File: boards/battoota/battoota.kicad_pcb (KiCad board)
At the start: 2 copper layers, 122.6 x 88.9 mm, 38 parts

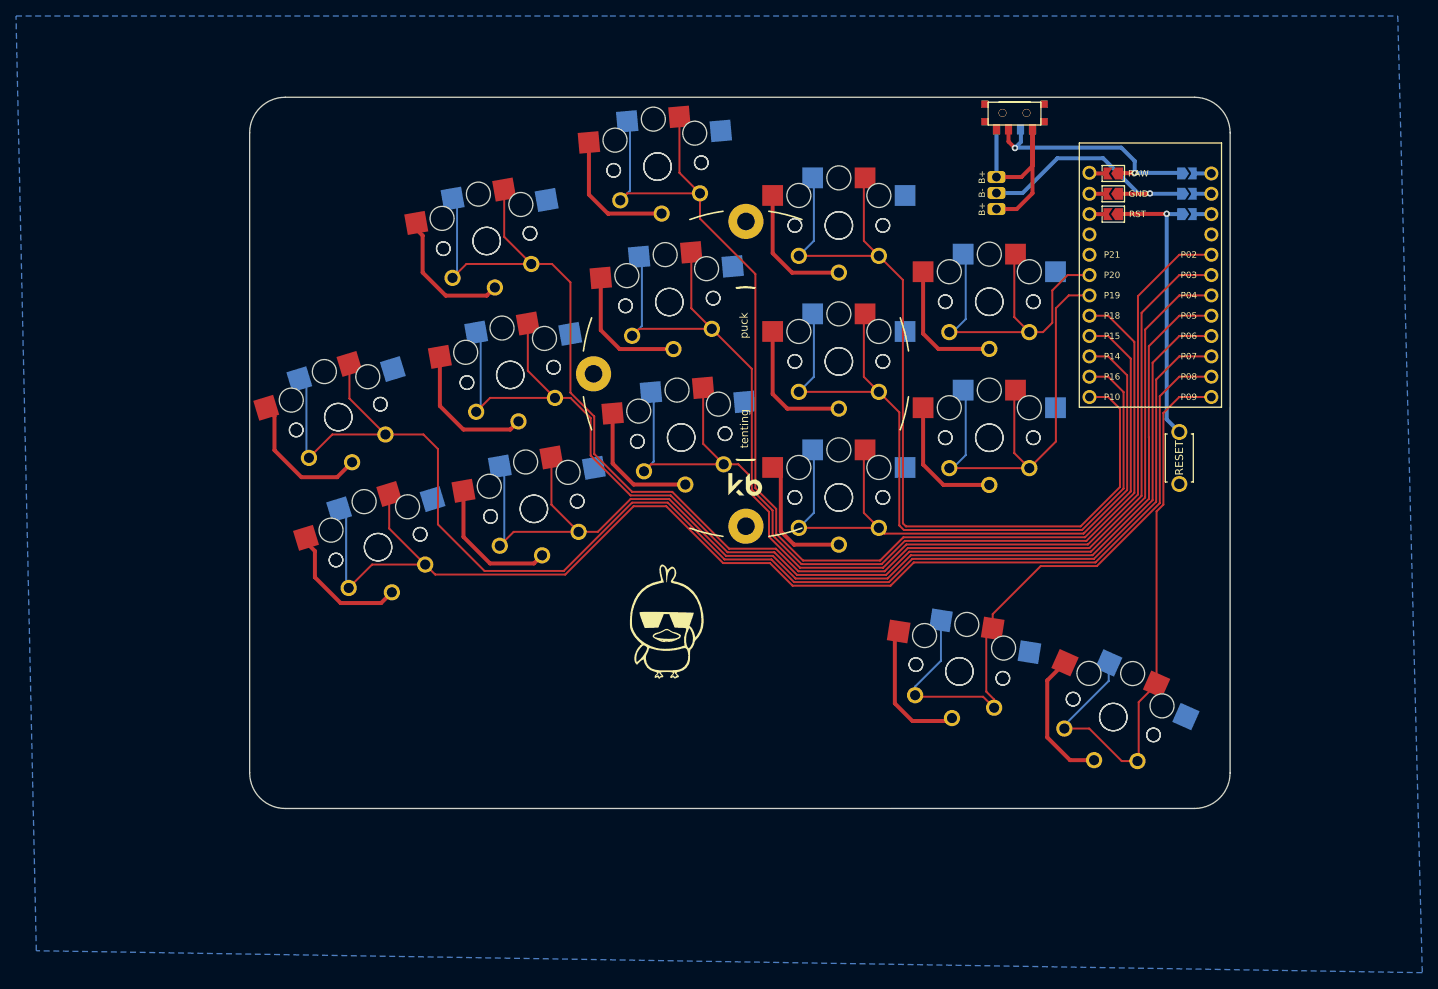
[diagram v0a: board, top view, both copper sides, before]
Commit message: battoota clean up
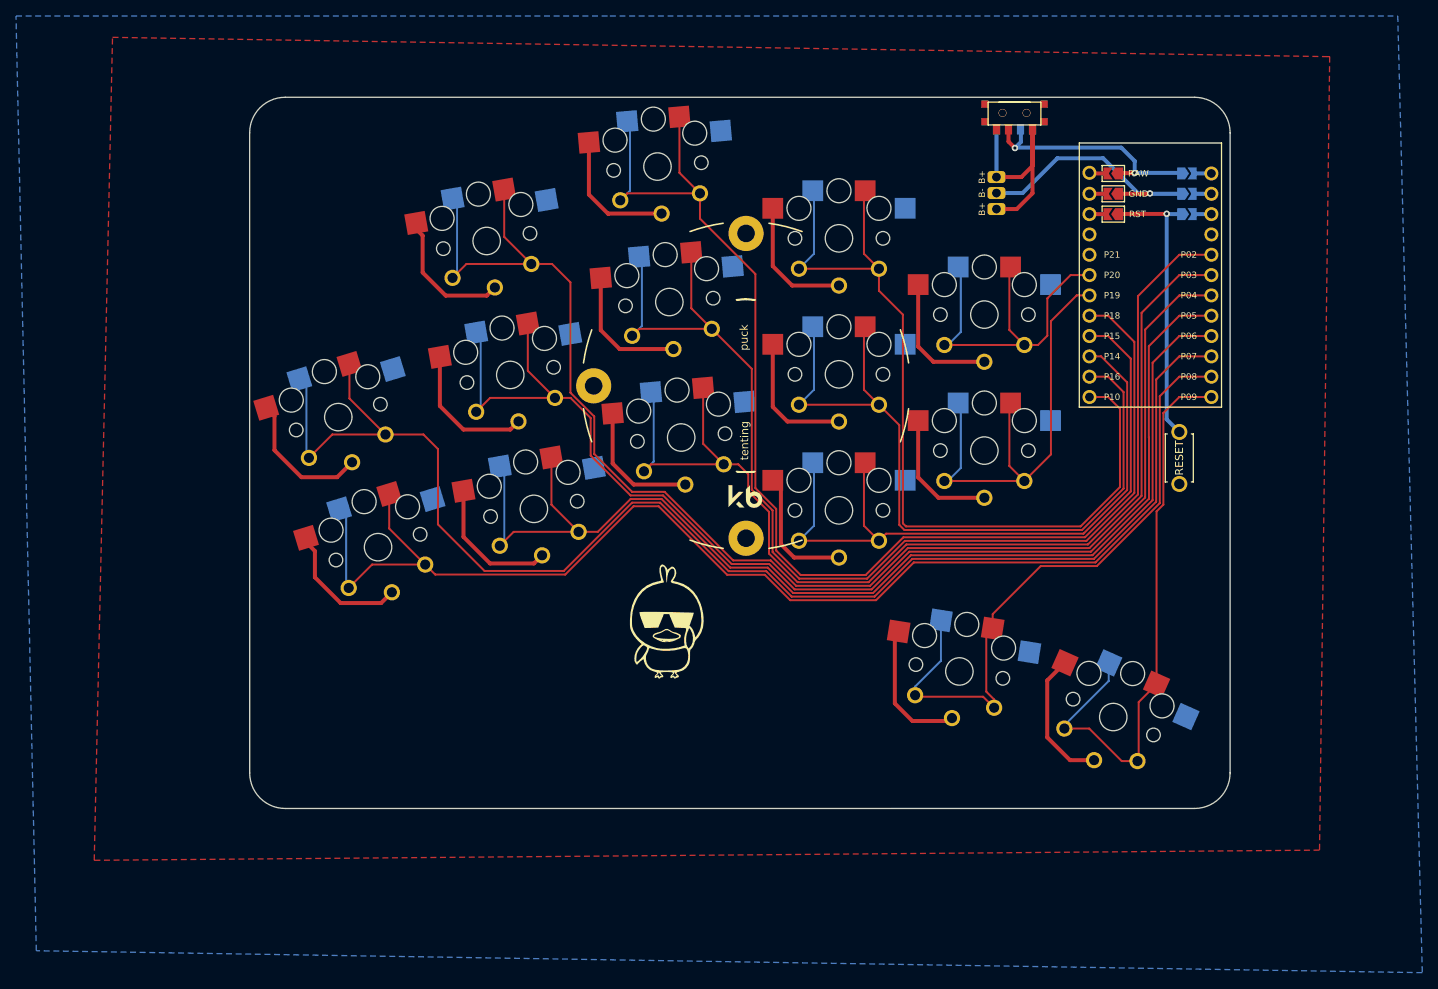
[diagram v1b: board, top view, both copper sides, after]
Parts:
- removed S10, S12, S14, S16, S18, S20, S22, S24, S28, S30, S32, S34, S4, S6, S8: , PG1350
- S11, S13, S15, S17, S19, S21, S23, S27, S29, S3, S31, S33, S5, S7, S9: footprint PG1350 -> Alaa:choc_hotswap_key
- moved S27 1.72 mm to (133.6, -78.5)
- moved S29 1.72 mm to (133.6, -95.5)
- moved S19 1.61 mm to (115.4, -71.1)
- moved S21 1.61 mm to (115.4, -88.1)
- moved S23 1.61 mm to (115.4, -105.1)
- moved REF** 1.50 mm to (103.8, -86.6)
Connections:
- S11 pad : P3 -> (no net)
- S13 pad : P2 -> (no net)
- S27 pad : P19 -> (no net)
- S29 pad : P20 -> (no net)
- S7 pad : P5 -> (no net)
- S9 pad : P4 -> (no net)
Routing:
- net P2: track 131.6 -> 134.3 mm
- net P15: track 150.2 -> 152.9 mm
- net P18: track 136.7 -> 139.4 mm
- net P16: track 96.8 -> 95.1 mm
- net P20: track 43.9 -> 45.6 mm
- net P10: track 109.7 -> 108.1 mm
- net P7: track 159.0 -> 160.5 mm
- net P6: track 178.1 -> 179.6 mm
- net P4: track 152.4 -> 153.9 mm
- net P3: track 172.1 -> 173.6 mm
- net P5: track 141.4 -> 142.9 mm
- net P19: track 57.7 -> 58.9 mm
- added copper zone on F.Cu, net (none)
